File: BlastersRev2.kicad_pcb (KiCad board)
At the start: 2 copper layers, 204.8 x 146.8 mm, 62 parts, among them U1 ProMicro

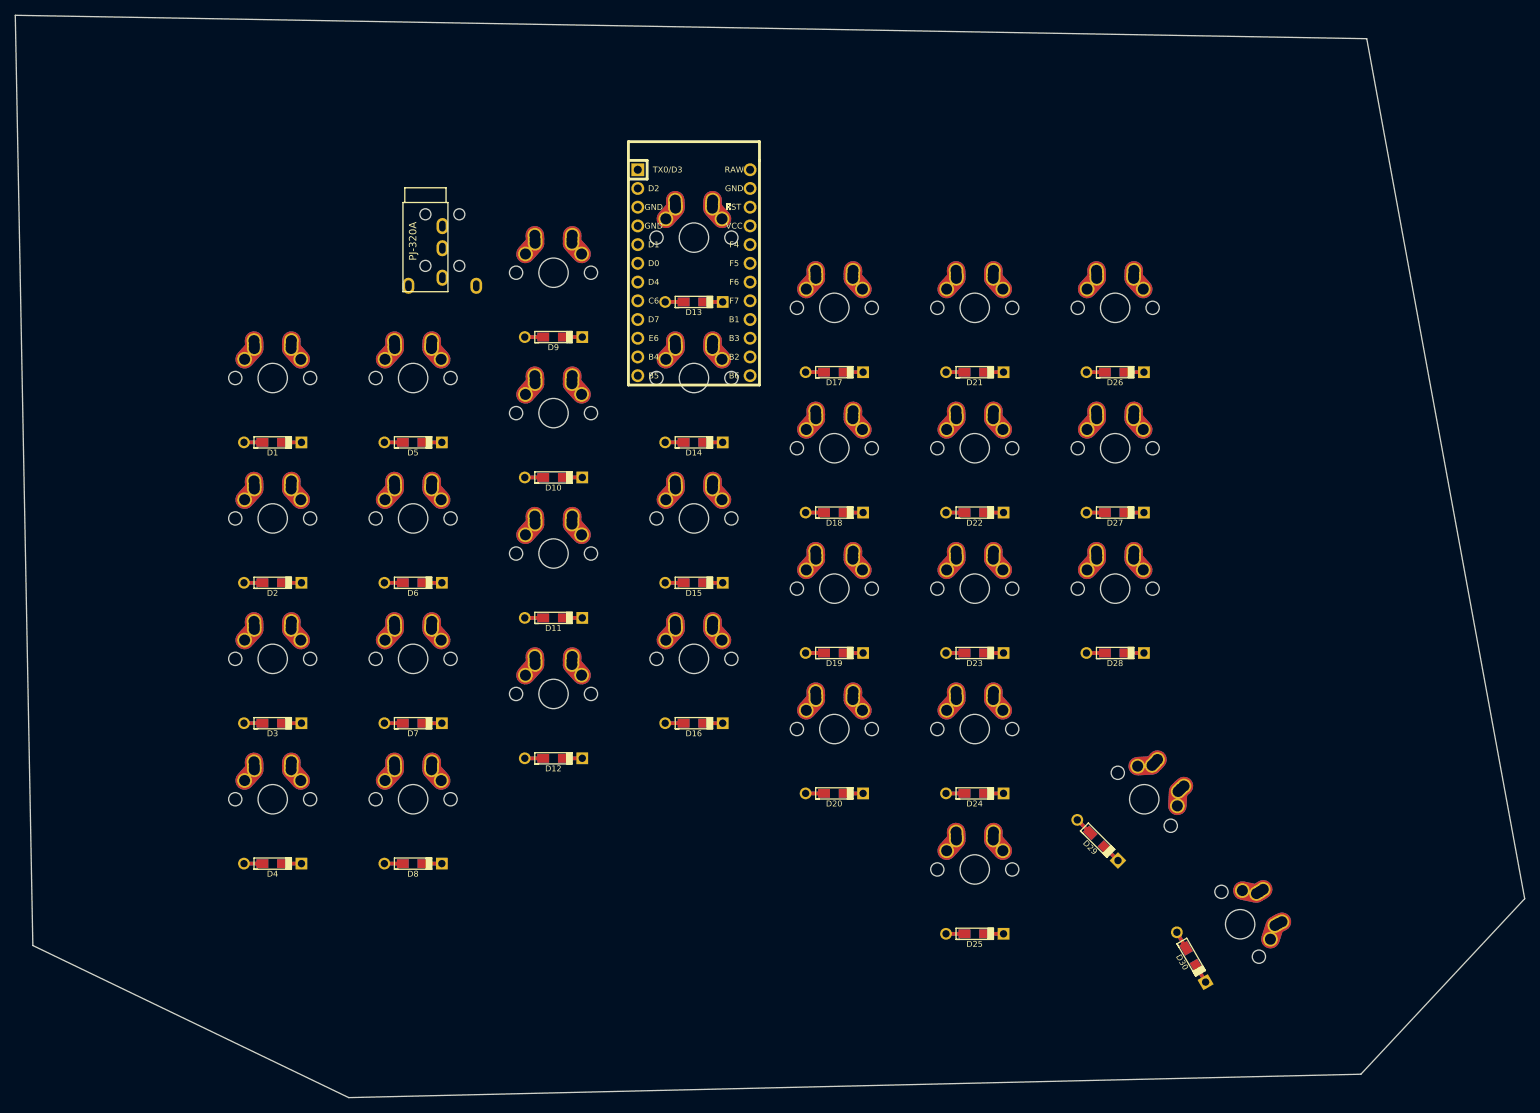
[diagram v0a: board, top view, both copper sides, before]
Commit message: Done!
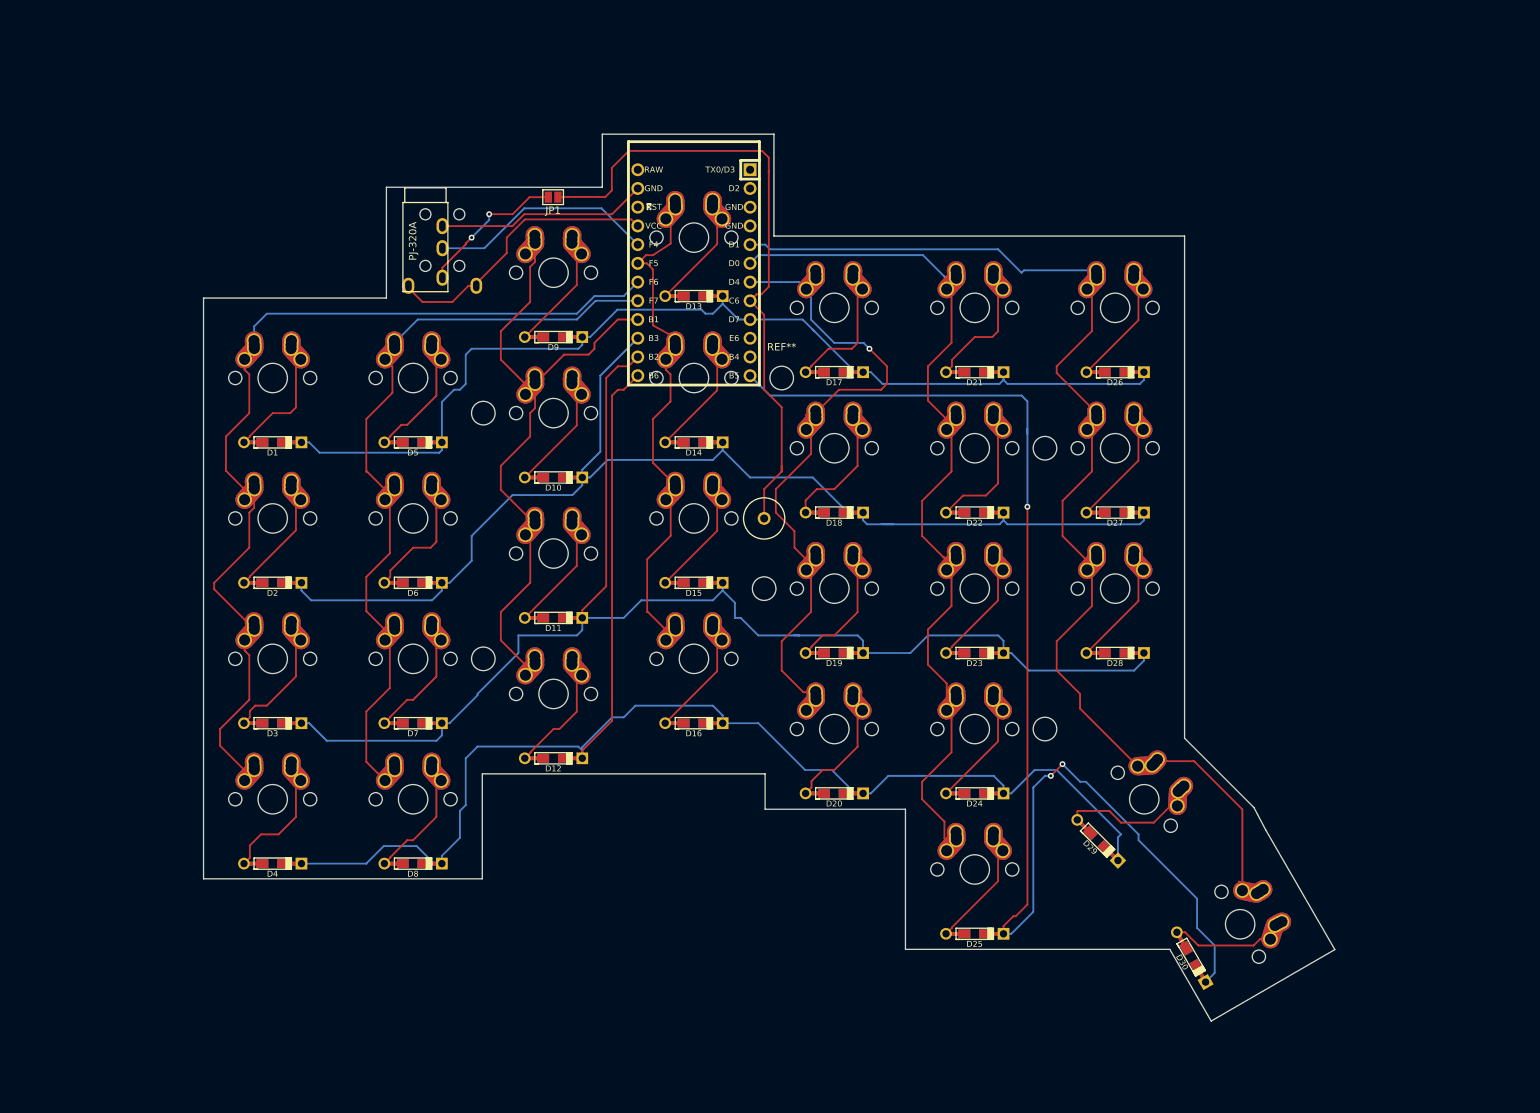
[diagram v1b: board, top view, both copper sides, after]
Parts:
- removed the REF** at (89.7, 61.9)
- added ?: MountingHole_3.2mm_M3, MountingHole:MountingHole_3.2mm_M3, F.Cu at (171.4, 95.2)
- added ?: MountingHole_3.2mm_M3, MountingHole:MountingHole_3.2mm_M3, F.Cu at (171.4, 133.3)
- added ?: MountingHole_3.2mm_M3, MountingHole:MountingHole_3.2mm_M3, F.Cu at (133.3, 114.3)
- added ?: MountingHole_3.2mm_M3, MountingHole:MountingHole_3.2mm_M3, F.Cu at (95.2, 123.8)
- added ?: MountingHole_3.2mm_M3, MountingHole:MountingHole_3.2mm_M3, F.Cu at (95.2, 90.5)
- added J1: AudioJack4_Ground, Keebio-Parts:TRRS-PJ-320A-dual, F.Cu at (89.7, 61.9)
- added JP1: Jumper, Jumper:SolderJumper-2_P1.3mm_Open_Pad1.0x1.5mm, F.Cu at (104.7, 61.2)
- added REF**: MountingHole_3.2mm_M3, MountingHole:MountingHole_3.2mm_M3, F.Cu at (135.7, 85.7)
- added U4: , Keebio-Parts:MountingHole, F.Cu at (133.3, 104.8)
- U1: moved to B.Cu
- moved D13 0.79 mm to (123.8, 74.6)
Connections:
- net Net-(U1-Pad21) renamed CommVcc
- net Net-(U1-Pad23) renamed CommGnd
- net Net-(U1-Pad3) renamed RGBGnd
- U1 pad 12: Net-(U1-Pad12) -> Row4
- U1 pad 13: Net-(U1-Pad13) -> Row3
- U1 pad 14: Net-(U1-Pad14) -> Row2
- U1 pad 15: Net-(U1-Pad15) -> Row1
- U1 pad 16: Net-(U1-Pad16) -> Col2
- U1 pad 17: Net-(U1-Pad17) -> Col1
- U1 pad 18: Net-(U1-Pad18) -> Col0
- U1 pad 19: Net-(U1-Pad19) -> Col3
- U1 pad 20: Net-(U1-Pad20) -> Comm
- U1 pad 5: Net-(U1-Pad5) -> Col6
- U1 pad 6: Net-(U1-Pad6) -> Col5
- U1 pad 7: Net-(U1-Pad7) -> Col4
- U1 pad 8: Net-(U1-Pad8) -> RGBCommBreakout
- U1 pad 9: Net-(U1-Pad9) -> Row0
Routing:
- net Row3: track 0.00 -> 203.6 mm
- net Row4: track 0.00 -> 180.1 mm, vias 0 -> 3
- net Row2: track 0.00 -> 179.6 mm
- net Row1: track 0.00 -> 159.6 mm
- net Col6: track 0.00 -> 156.7 mm
- net Row0: track 0.00 -> 139.1 mm
- net Col0: track 0.00 -> 124.2 mm
- net Col5: track 0.00 -> 118.0 mm
- net Col1: track 0.00 -> 100.8 mm
- net RGBCommBreakout: track 0.00 -> 87.5 mm
- net Col2: track 0.00 -> 87.4 mm
- net Col4: track 0.00 -> 86.7 mm, vias 0 -> 1
- net Col3: track 0.00 -> 67.8 mm
- net CommVcc: track 0.00 -> 38.9 mm
- net Comm: track 0.00 -> 30.8 mm
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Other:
- board size 204.8 x 146.8 mm -> 153.5 x 120.3 mm
